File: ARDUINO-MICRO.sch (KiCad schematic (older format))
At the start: 48 parts, among them P1 RC_IN, P2 ICSP, P3 USB-MICRO, P4 RS232, SW1 SW_PUSH, U1 ATmega32U4, U2 ADM3101E, Y1 16MHz

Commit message: Update
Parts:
- F1: value 0.5A -> 0.2A; footprint Fuse:Fuse_1812_4532Metric -> Fuse:Fuse_1206_3216Metric; ProviderCode 652-MF-MSMF050-2 -> 652-MF-NSMF020X-2; manf# MF-MSMF050-2 -> MF-NSMF020X-2
- JP1: symbol Jumper:Jumper_3_Bridged12 -> Driverino-rescue:Jumper_3_Bridged12-Jumper
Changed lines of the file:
@@
 AR Path="/614792E0/614921EC" Ref="F1"  Part="1"
 F 0 "F1" H 12925 5492 40  0000 C CNN
-F 1 "0.5A " H 12925 5416 40  0000 C CNN
-F 2 "Fuse:Fuse_1812_4532Metric" H 12925 5275 60  0001 C CNN
+F 1 "0.2A " H 12925 5416 40  0000 C CNN
+F 2 "Fuse:Fuse_1206_3216Metric" H 12925 5275 60  0001 C CNN
 F 3 "" H 12925 5275 60  0001 C CNN
 F 4 "Bourns" H 12925 5275 50  0001 C CNN "Manufacturer"
-F 5 "" H 12925 5275 50  0001 C CNN "P/N"
-F 6 "652-MF-MSMF050-2" H 12925 5275 50  0001 C CNN "ProviderCode"
-F 7 "Mouser" H 12925 5275 50  0001 C CNN "Provider"
-F 8 "MF-MSMF050-2" H 12925 5275 50  0001 C CNN "manf#"
-F 9 "" H 12925 5275 50  0001 C CNN "Productor"
+F 5 "652-MF-NSMF020X-2" H 12925 5275 50  0001 C CNN "ProviderCode"
+F 6 "Mouser" H 12925 5275 50  0001 C CNN "Provider"
+F 7 "MF-NSMF020X-2" H 12925 5275 50  0001 C CNN "manf#"
+F 8 "" H 12925 5275 50  0001 C CNN "Productor"
 	1    12925 5275
 	1    0    0    -1
@@
 $EndComp
 $Comp
-L Jumper:Jumper_3_Bridged12 JP?
+L Driverino-rescue:Jumper_3_Bridged12-Jumper JP?
 U 1 1 609E3044
 P 13900 2075

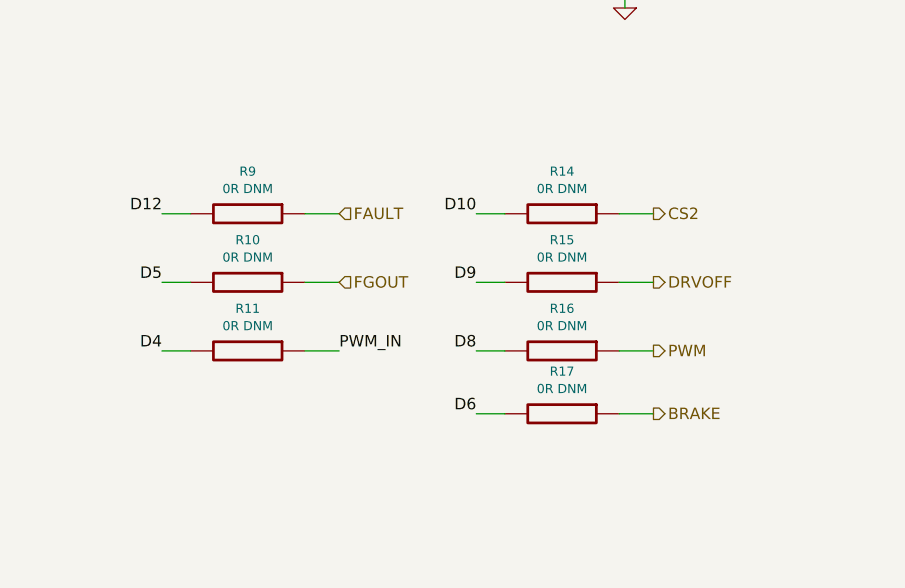
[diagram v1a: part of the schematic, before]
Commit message: Update
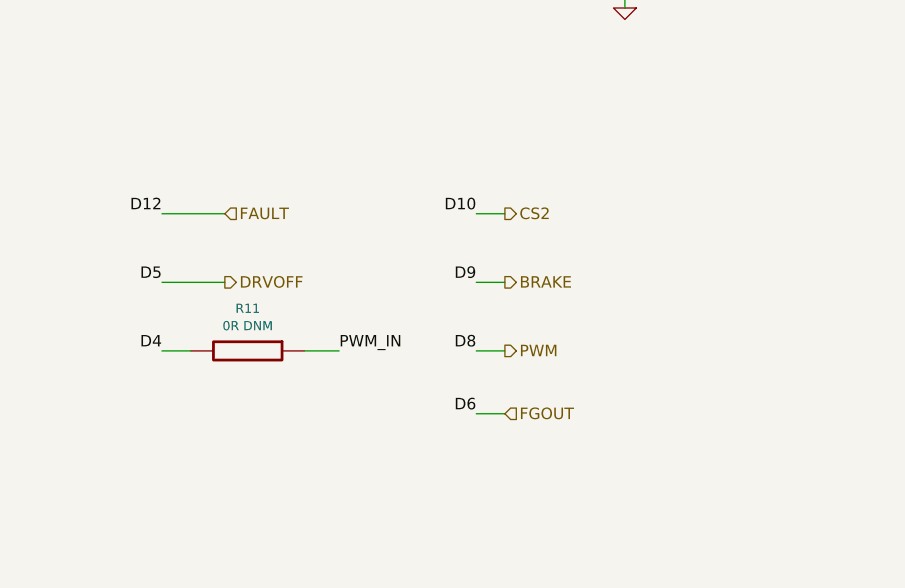
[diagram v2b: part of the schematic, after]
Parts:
- removed R10, R14, R15, R16, R17, R9: 0R DNM, Resistor_SMD:R_0402_1005Metric, symbol Driverino-rescue:R-device
- D4: footprint Diode_SMD:D_SOD-123 -> Diode_SMD:D_0603_1608Metric; ProviderCode 771-BZT52-C4V7X -> 771-BZX884S-C5V1YL; manf# BZT52-C4V7X -> BZX884S-C5V1YL
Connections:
- net D10 is gone; now on net CS2: U1.30 (PB6)
- net D12 is gone; now on net FAULT: U1.26 (PD6)
- net D5 is gone; now on net DRVOFF: U1.31 (PC6)
- net D6 is gone; now on net FGOUT: U1.27 (PD7)
- net D8 is gone; now on net PWM: U1.28 (PB4)
- net D9 is gone; now on net BRAKE: U1.29 (PB5)
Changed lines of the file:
@@
 Text Label 13250 8525 2    50   ~ 0
 D6
-Text HLabel 12650 7950 2    50   Input ~ 0
+Text HLabel 13375 8525 2    50   Input ~ 0
 FGOUT
-$Comp
-L Driverino-rescue:R-device R?
-U 1 1 61658E20
-P 13625 7650
-AR Path="/61658E20" Ref="R?"  Part="1"
-AR Path="/614792E0/61658E20" Ref="R14"  Part="1"
-F 0 "R14" V 13440 7650 40  0000 C CNN
-F 1 "0R DNM" V 13516 7650 40  0000 C CNN
-F 2 "Resistor_SMD:R_0402_1005Metric" V 13555 7650 30  0001 C CNN
-F 3 "" H 13625 7650 30  0000 C CNN
-F 4 "Mouser" H 13625 7650 50  0001 C CNN "Provider"
-F 5 "Vishay" H 13625 7650 50  0001 C CNN "Manufacturer"
-F 6 "71-RCC04020000Z0ED" H 13625 7650 50  0001 C CNN "ProviderCode"
-F 7 "RCC04020000Z0ED" H 13625 7650 50  0001 C CNN "manf#"
-	1    13625 7650
-	0    1    1    0
-$EndComp
-Wire Wire Line
-	13250 7650 13375 7650
-Wire Wire Line
-	13875 7650 14025 7650
-Text HLabel 14025 7650 2    50   Output ~ 0
+Text HLabel 13375 7650 2    50   Output ~ 0
 CS2
-$Comp
-L Driverino-rescue:R-device R?
-U 1 1 61663BE3
-P 13625 7950
-AR Path="/61663BE3" Ref="R?"  Part="1"
-AR Path="/614792E0/61663BE3" Ref="R15"  Part="1"
-F 0 "R15" V 13440 7950 40  0000 C CNN
-F 1 "0R DNM" V 13516 7950 40  0000 C CNN
-F 2 "Resistor_SMD:R_0402_1005Metric" V 13555 7950 30  0001 C CNN
-F 3 "" H 13625 7950 30  0000 C CNN
-F 4 "Mouser" H 13625 7950 50  0001 C CNN "Provider"
-F 5 "Vishay" H 13625 7950 50  0001 C CNN "Manufacturer"
-F 6 "71-RCC04020000Z0ED" H 13625 7950 50  0001 C CNN "ProviderCode"
-F 7 "RCC04020000Z0ED" H 13625 7950 50  0001 C CNN "manf#"
-	1    13625 7950
-	0    1    1    0
-$EndComp
 Wire Wire Line
 	13250 7950 13375 7950
-Wire Wire Line
-	13875 7950 14025 7950
-Text HLabel 14025 7950 2    50   Output ~ 0
+Text HLabel 12150 7950 2    50   Output ~ 0
 DRVOFF
-$Comp
-L Driverino-rescue:R-device R?
-U 1 1 61663BF1
-P 13625 8250
-AR Path="/61663BF1" Ref="R?"  Part="1"
-AR Path="/614792E0/61663BF1" Ref="R16"  Part="1"
-F 0 "R16" V 13440 8250 40  0000 C CNN
-F 1 "0R DNM" V 13516 8250 40  0000 C CNN
-F 2 "Resistor_SMD:R_0402_1005Metric" V 13555 8250 30  0001 C CNN
-F 3 "" H 13625 8250 30  0000 C CNN
-F 4 "Mouser" H 13625 8250 50  0001 C CNN "Provider"
-F 5 "Vishay" H 13625 8250 50  0001 C CNN "Manufacturer"
-F 6 "71-RCC04020000Z0ED" H 13625 8250 50  0001 C CNN "ProviderCode"
-F 7 "RCC04020000Z0ED" H 13625 8250 50  0001 C CNN "manf#"
-	1    13625 8250
-	0    1    1    0
-$EndComp
 Wire Wire Line
 	13250 8250 13375 8250
-Wire Wire Line
-	13875 8250 14025 8250
-Text HLabel 14025 8250 2    50   Output ~ 0
+Text HLabel 13375 8250 2    50   Output ~ 0
 PWM
-$Comp
-L Driverino-rescue:R-device R?
-U 1 1 6166E2E1
-P 13625 8525
-AR Path="/6166E2E1" Ref="R?"  Part="1"
-AR Path="/614792E0/6166E2E1" Ref="R17"  Part="1"
-F 0 "R17" V 13440 8525 40  0000 C CNN
-F 1 "0R DNM" V 13516 8525 40  0000 C CNN
-F 2 "Resistor_SMD:R_0402_1005Metric" V 13555 8525 30  0001 C CNN
-F 3 "" H 13625 8525 30  0000 C CNN
-F 4 "Mouser" H 13625 8525 50  0001 C CNN "Provider"
-F 5 "Vishay" H 13625 8525 50  0001 C CNN "Manufacturer"
-F 6 "71-RCC04020000Z0ED" H 13625 8525 50  0001 C CNN "ProviderCode"
-F 7 "RCC04020000Z0ED" H 13625 8525 50  0001 C CNN "manf#"
-	1    13625 8525
-	0    1    1    0
-$EndComp
 Wire Wire Line
 	13250 8525 13375 8525
-Wire Wire Line
-	13875 8525 14025 8525
-Text HLabel 14025 8525 2    50   Output ~ 0
+Text HLabel 13375 7950 2    50   Output ~ 0
 BRAKE
-Text HLabel 12650 7650 2    50   Input ~ 0
+Text HLabel 12150 7650 2    50   Input ~ 0
 FAULT
 Wire Wire Line
@@
 Text Label 11875 7650 2    50   ~ 0
 D12
-Wire Wire Line
-	12500 7650 12650 7650
-Wire Wire Line
-	11875 7650 12000 7650
-$Comp
-L Driverino-rescue:R-device R?
-U 1 1 616A9031
-P 12250 7650
-AR Path="/616A9031" Ref="R?"  Part="1"
-AR Path="/614792E0/616A9031" Ref="R9"  Part="1"
-F 0 "R9" V 12065 7650 40  0000 C CNN
-F 1 "0R DNM" V 12141 7650 40  0000 C CNN
-F 2 "Resistor_SMD:R_0402_1005Metric" V 12180 7650 30  0001 C CNN
-F 3 "" H 12250 7650 30  0000 C CNN
-F 4 "Mouser" H 12250 7650 50  0001 C CNN "Provider"
-F 5 "Vishay" H 12250 7650 50  0001 C CNN "Manufacturer"
-F 6 "71-RCC04020000Z0ED" H 12250 7650 50  0001 C CNN "ProviderCode"
-F 7 "RCC04020000Z0ED" H 12250 7650 50  0001 C CNN "manf#"
-	1    12250 7650
-	0    1    1    0
-$EndComp
-Wire Wire Line
-	12500 7950 12650 7950
-Wire Wire Line
-	11875 7950 12000 7950
-$Comp
-L Driverino-rescue:R-device R?
-U 1 1 61643BD7
-P 12250 7950
-AR Path="/61643BD7" Ref="R?"  Part="1"
-AR Path="/614792E0/61643BD7" Ref="R10"  Part="1"
-F 0 "R10" V 12065 7950 40  0000 C CNN
-F 1 "0R DNM" V 12141 7950 40  0000 C CNN
-F 2 "Resistor_SMD:R_0402_1005Metric" V 12180 7950 30  0001 C CNN
-F 3 "" H 12250 7950 30  0000 C CNN
-F 4 "Mouser" H 12250 7950 50  0001 C CNN "Provider"
-F 5 "Vishay" H 12250 7950 50  0001 C CNN "Manufacturer"
-F 6 "71-RCC04020000Z0ED" H 12250 7950 50  0001 C CNN "ProviderCode"
-F 7 "RCC04020000Z0ED" H 12250 7950 50  0001 C CNN "manf#"
-	1    12250 7950
-	0    1    1    0
-$EndComp
 Text Label 11875 7950 2    50   ~ 0
 D5
@@
 F 0 "D4" V 8405 9556 40  0000 R CNN
 F 1 "VZ=5V" V 8337 9556 30  0000 R CNN
-F 2 "Diode_SMD:D_SOD-123" V 8325 9550 60  0001 R CNN
+F 2 "Diode_SMD:D_0603_1608Metric" V 8325 9550 60  0001 R CNN
 F 3 "" H 8375 9625 60  0000 C CNN
 F 4 "Mouser" H 8375 9625 50  0001 C CNN "Provider"
 F 5 "" H 8375 9625 50  0001 C CNN "Code"
-F 6 "" H 8375 9625 50  0001 C CNN "P/N"
-F 7 "" H 8375 9625 50  0001 C CNN "Productor"
-F 8 "BZT52-C4V7X" H 8375 9625 50  0001 C CNN "manf#"
-F 9 "Nexperia" H 8375 9625 50  0001 C CNN "Manufacturer"
-F 10 "771-BZT52-C4V7X" H 8375 9625 50  0001 C CNN "ProviderCode"
+F 6 "" H 8375 9625 50  0001 C CNN "Productor"
+F 7 "BZX884S-C5V1YL" H 8375 9625 50  0001 C CNN "manf#"
+F 8 "Nexperia" H 8375 9625 50  0001 C CNN "Manufacturer"
+F 9 "771-BZX884S-C5V1YL" H 8375 9625 50  0001 C CNN "ProviderCode"
 	1    8375 9625
 	0    -1   -1   0
@@
 Text Label 11875 8250 2    50   ~ 0
 D4
+Wire Wire Line
+	11875 7950 12150 7950
+Wire Wire Line
+	13250 7650 13375 7650
+Wire Wire Line
+	11875 7650 12150 7650
 $EndSCHEMATC

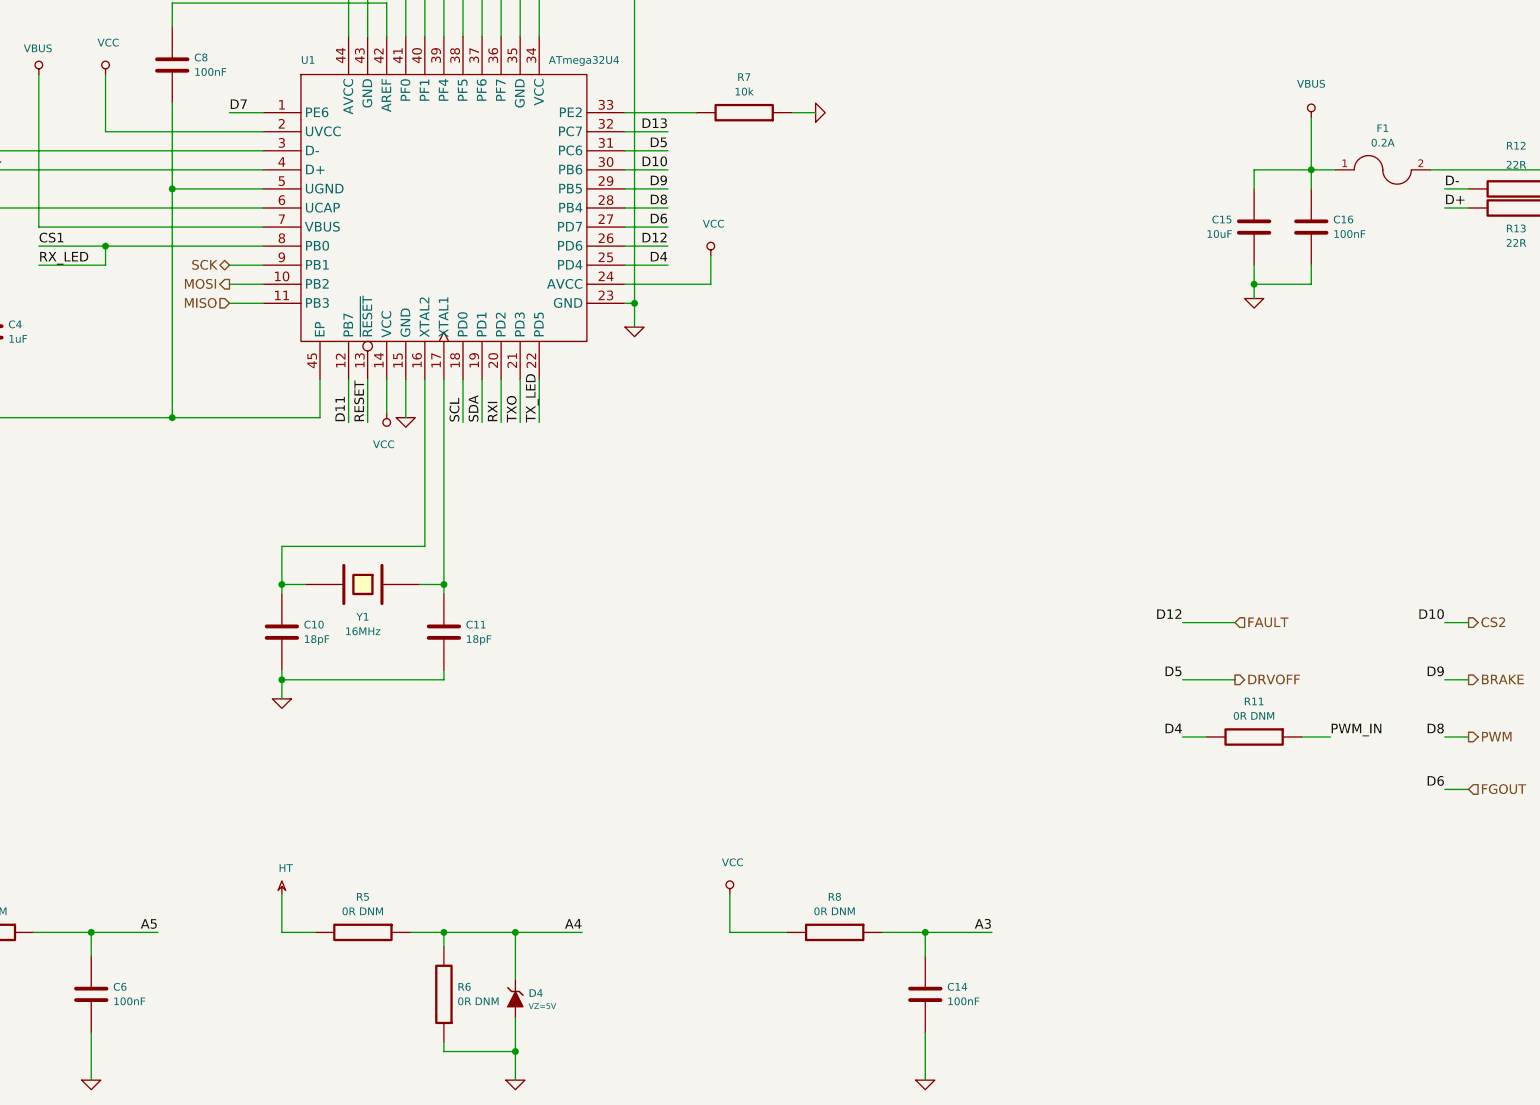
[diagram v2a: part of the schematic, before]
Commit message: Modified F1
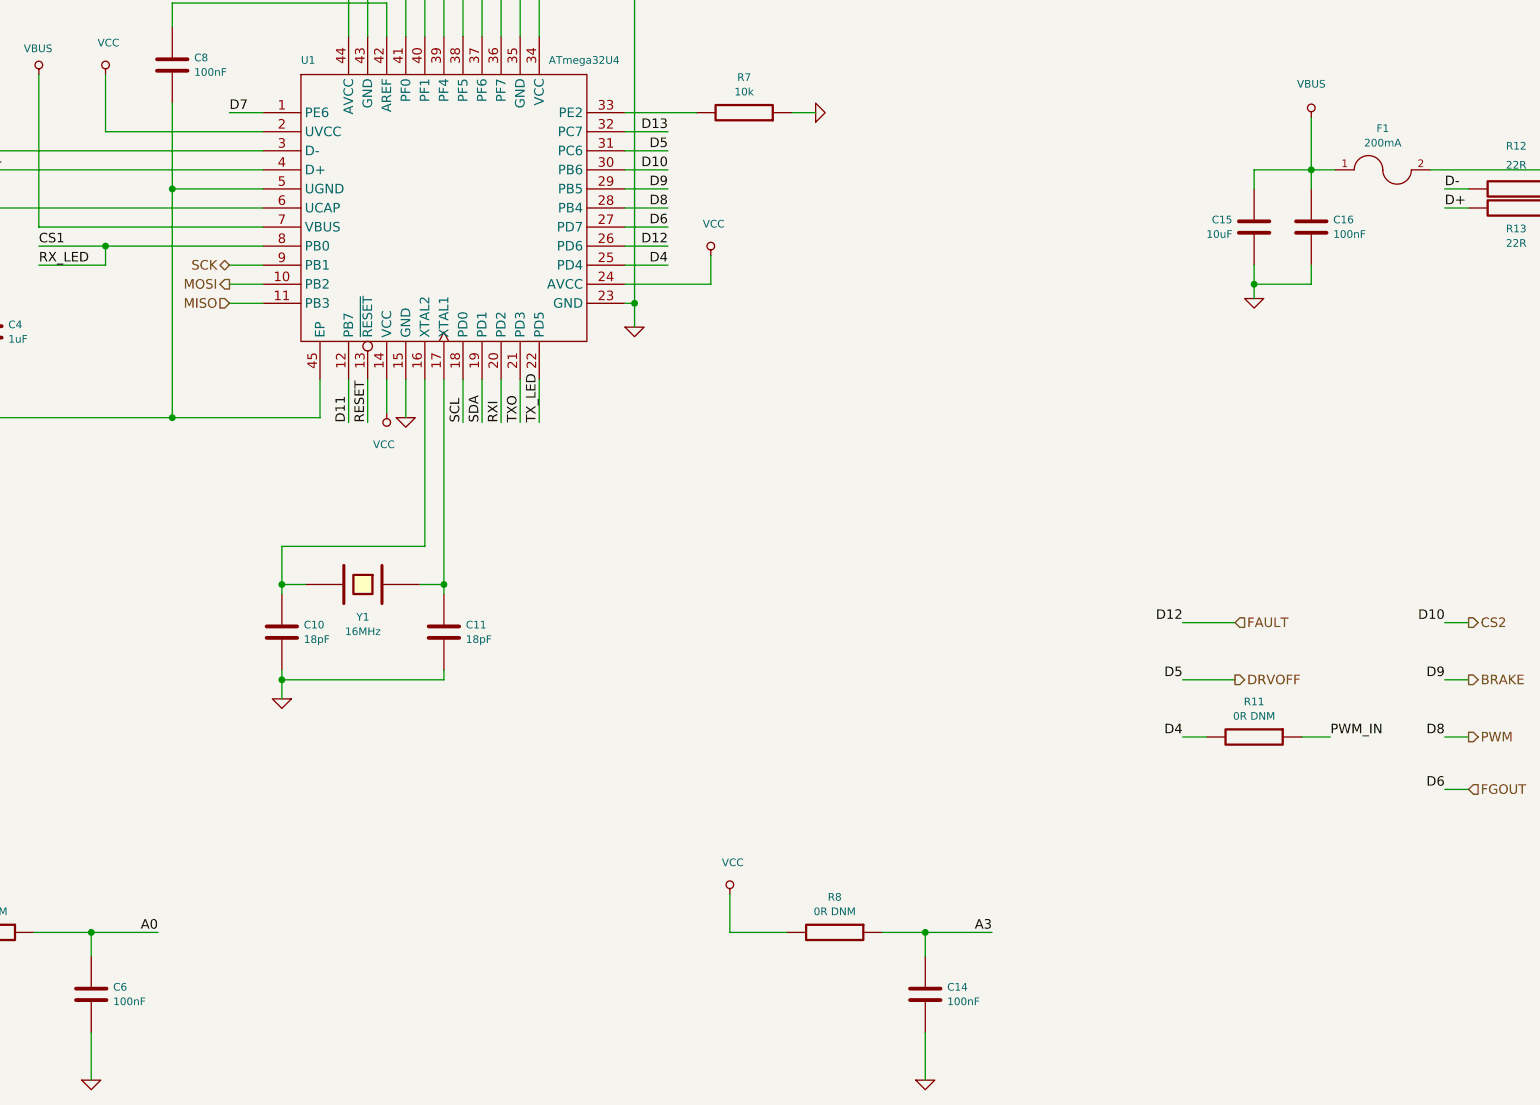
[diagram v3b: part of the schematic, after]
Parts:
- removed D4: VZ=5V, Diode_SMD:D_0603_1608Metric, symbol Driverino-rescue:ZENERsmall-device
- removed R5, R6: 0R DNM, Resistor_SMD:R_0402_1005Metric, symbol Driverino-rescue:R-device
- F1: value 0.2A -> 200mA; footprint Fuse:Fuse_1206_3216Metric -> Fuse:Fuse_0402_1005Metric; ProviderCode 652-MF-NSMF020X-2 -> 652-MF-ASML020/6-2; manf# MF-NSMF020X-2 -> MF-ASML020/6-2
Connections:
- net A0: now also C6.2, R4.1
- net A5: no longer C6.2, R4.1
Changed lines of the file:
@@
 Wire Wire Line
 	14225 4650 14050 4650
-Text Label 6500 9275 2    50   ~ 0
-A5
 Wire Wire Line
 	5150 9275 5350 9275
@@
 AR Path="/614792E0/614921EC" Ref="F1"  Part="1"
 F 0 "F1" H 12925 5492 40  0000 C CNN
-F 1 "0.2A " H 12925 5416 40  0000 C CNN
-F 2 "Fuse:Fuse_1206_3216Metric" H 12925 5275 60  0001 C CNN
+F 1 "200mA" H 12925 5416 40  0000 C CNN
+F 2 "Fuse:Fuse_0402_1005Metric" H 12925 5275 60  0001 C CNN
 F 3 "" H 12925 5275 60  0001 C CNN
 F 4 "Bourns" H 12925 5275 50  0001 C CNN "Manufacturer"
-F 5 "652-MF-NSMF020X-2" H 12925 5275 50  0001 C CNN "ProviderCode"
+F 5 "652-MF-ASML020/6-2" H 12925 5275 50  0001 C CNN "ProviderCode"
 F 6 "Mouser" H 12925 5275 50  0001 C CNN "Provider"
-F 7 "MF-NSMF020X-2" H 12925 5275 50  0001 C CNN "manf#"
+F 7 "MF-ASML020/6-2" H 12925 5275 50  0001 C CNN "manf#"
 F 8 "" H 12925 5275 50  0001 C CNN "Productor"
 	1    12925 5275
@@
 Wire Wire Line
 	12550 5375 12550 5275
-Wire Wire Line
-	7150 9075 7150 9275
-$Comp
-L power:HT #PWR?
-U 1 1 614922C9
-P 7150 9075
-AR Path="/614922C9" Ref="#PWR?"  Part="1"
-AR Path="/614792E0/614922C9" Ref="#PWR013"  Part="1"
-F 0 "#PWR013" H 7150 9195 20  0001 C CNN
-F 1 "HT" H 7170 9211 40  0000 C CNN
-F 2 "" H 7150 9075 50  0001 C CNN
-F 3 "" H 7150 9075 50  0001 C CNN
-	1    7150 9075
-	1    0    0    -1
-$EndComp
 Text Label 14050 4650 0    50   ~ 0
 RESET
@@
 Wire Wire Line
 	12250 5875 12250 5950
-Text Label 10875 9275 2    50   ~ 0
-A3
 Wire Wire Line
 	9500 9275 9800 9275
@@
 	12250 5875 12550 5875
 Wire Wire Line
-	8375 9900 8375 10050
-Connection ~ 8375 9900
-Wire Wire Line
-	8000 9900 8375 9900
-Wire Wire Line
-	8000 9850 8000 9900
-Wire Wire Line
-	8000 9275 8375 9275
-Connection ~ 8000 9275
-Wire Wire Line
-	8000 9350 8000 9275
-Connection ~ 8375 9275
-Wire Wire Line
-	8375 9275 8725 9275
-$Comp
-L Driverino-rescue:R-device R?
-U 1 1 614920AF
-P 8000 9600
-AR Path="/614920AF" Ref="R?"  Part="1"
-AR Path="/614792E0/614920AF" Ref="R6"  Part="1"
-F 0 "R6" H 7929 9562 40  0000 R CNN
-F 1 "0R DNM" H 7929 9638 40  0000 R CNN
-F 2 "Resistor_SMD:R_0402_1005Metric" V 7930 9600 30  0001 C CNN
-F 3 "" H 8000 9600 30  0000 C CNN
-F 4 "Mouser" H 8000 9600 50  0001 C CNN "Provider"
-F 5 "Vishay" H 8000 9600 50  0001 C CNN "Manufacturer"
-F 6 "71-RCC04020000Z0ED" H 8000 9600 50  0001 C CNN "ProviderCode"
-F 7 "RCC04020000Z0ED" H 8000 9600 50  0001 C CNN "manf#"
-	1    8000 9600
-	-1   0    0    1
-$EndComp
-Wire Wire Line
-	8375 9725 8375 9900
-Wire Wire Line
-	8375 9275 8375 9525
-$Comp
-L Driverino-rescue:ZENERsmall-device D?
-U 1 1 6149209F
-P 8375 9625
-AR Path="/6149209F" Ref="D?"  Part="1"
-AR Path="/614792E0/6149209F" Ref="D4"  Part="1"
-F 0 "D4" V 8405 9556 40  0000 R CNN
-F 1 "VZ=5V" V 8337 9556 30  0000 R CNN
-F 2 "Diode_SMD:D_0603_1608Metric" V 8325 9550 60  0001 R CNN
-F 3 "" H 8375 9625 60  0000 C CNN
-F 4 "Mouser" H 8375 9625 50  0001 C CNN "Provider"
-F 5 "" H 8375 9625 50  0001 C CNN "Code"
-F 6 "" H 8375 9625 50  0001 C CNN "Productor"
-F 7 "BZX884S-C5V1YL" H 8375 9625 50  0001 C CNN "manf#"
-F 8 "Nexperia" H 8375 9625 50  0001 C CNN "Manufacturer"
-F 9 "771-BZX884S-C5V1YL" H 8375 9625 50  0001 C CNN "ProviderCode"
-	1    8375 9625
-	0    -1   -1   0
-$EndComp
-$Comp
-L Driverino-rescue:GND-power #PWR?
-U 1 1 61492093
-P 8375 10050
-AR Path="/61492093" Ref="#PWR?"  Part="1"
-AR Path="/614792E0/61492093" Ref="#PWR017"  Part="1"
-F 0 "#PWR017" H 8375 10050 30  0001 C CNN
-F 1 "GND" H 8375 9980 30  0001 C CNN
-F 2 "" H 8375 10050 50  0001 C CNN
-F 3 "" H 8375 10050 50  0001 C CNN
-	1    8375 10050
-	1    0    0    -1
-$EndComp
-Text Label 8725 9275 2    50   ~ 0
-A4
-Wire Wire Line
-	7150 9275 7325 9275
-Wire Wire Line
-	7825 9275 8000 9275
-$Comp
-L Driverino-rescue:R-device R?
-U 1 1 614920A8
-P 7575 9275
-AR Path="/614920A8" Ref="R?"  Part="1"
-AR Path="/614792E0/614920A8" Ref="R5"  Part="1"
-F 0 "R5" V 7390 9275 40  0000 C CNN
-F 1 "0R DNM" V 7466 9275 40  0000 C CNN
-F 2 "Resistor_SMD:R_0402_1005Metric" V 7505 9275 30  0001 C CNN
-F 3 "" H 7575 9275 30  0000 C CNN
-F 4 "Mouser" H 7575 9275 50  0001 C CNN "Provider"
-F 5 "Vishay" H 7575 9275 50  0001 C CNN "Manufacturer"
-F 6 "71-RCC04020000Z0ED" H 7575 9275 50  0001 C CNN "ProviderCode"
-F 7 "RCC04020000Z0ED" H 7575 9275 50  0001 C CNN "manf#"
-	1    7575 9275
-	0    1    1    0
-$EndComp
-Wire Wire Line
 	7350 6375 7350 6575
 Wire Wire Line
@@
 Wire Wire Line
 	11875 7650 12150 7650
+Text Label 10875 9275 2    50   ~ 0
+A3
+Text Label 6500 9275 2    50   ~ 0
+A0
 $EndSCHEMATC
